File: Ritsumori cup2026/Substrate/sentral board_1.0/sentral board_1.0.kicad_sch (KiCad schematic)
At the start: 9 parts, among them J1 Conn_02x10_Odd_Even, J2 Conn_02x05_Counter_Clockwise, J3 Conn_01x04_Socket, J4 Conn_01x05_Socket, J5 Conn_01x02_Socket, J6 Conn_01x02_Socket, J7 Conn_01x02_Socket, J8 Conn_01x02_Socket, J9 Conn_01x04_Socket

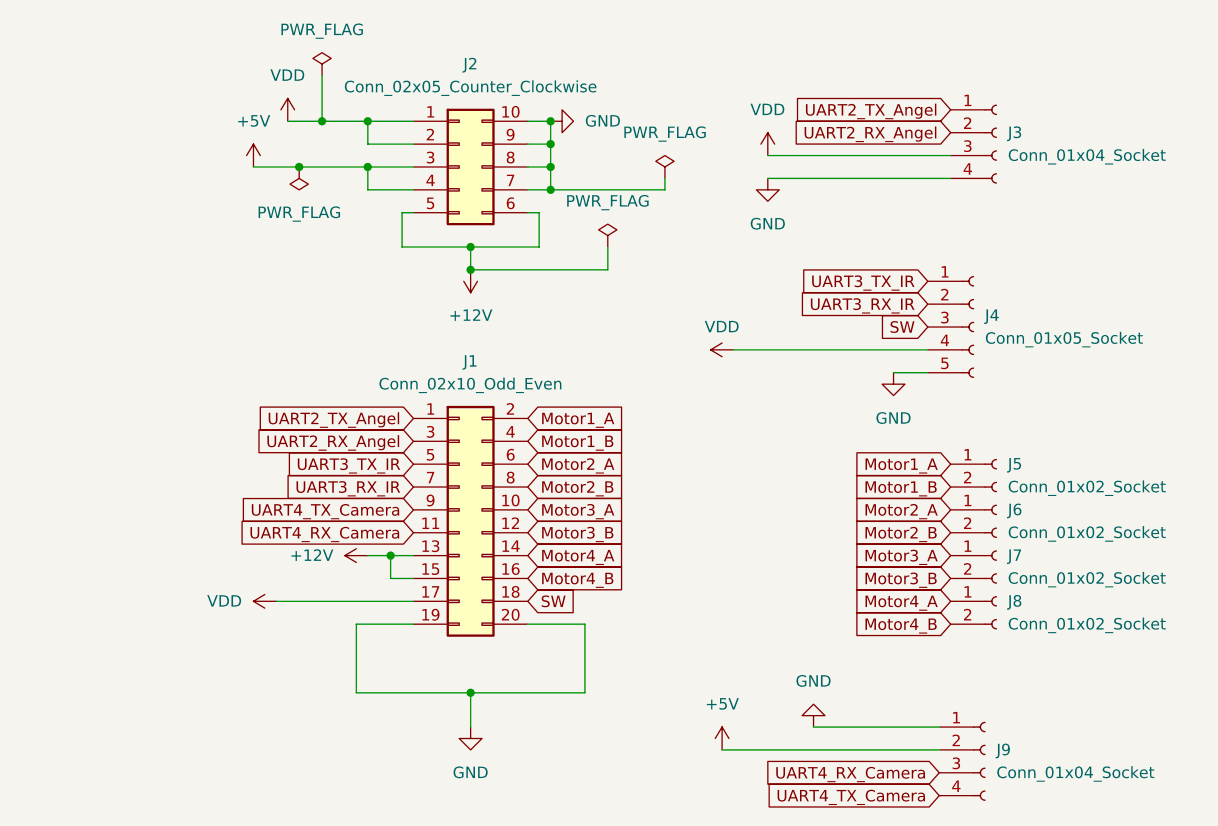
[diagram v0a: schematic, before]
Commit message: Auto Backup: 2026/02/19 18:25:14.96
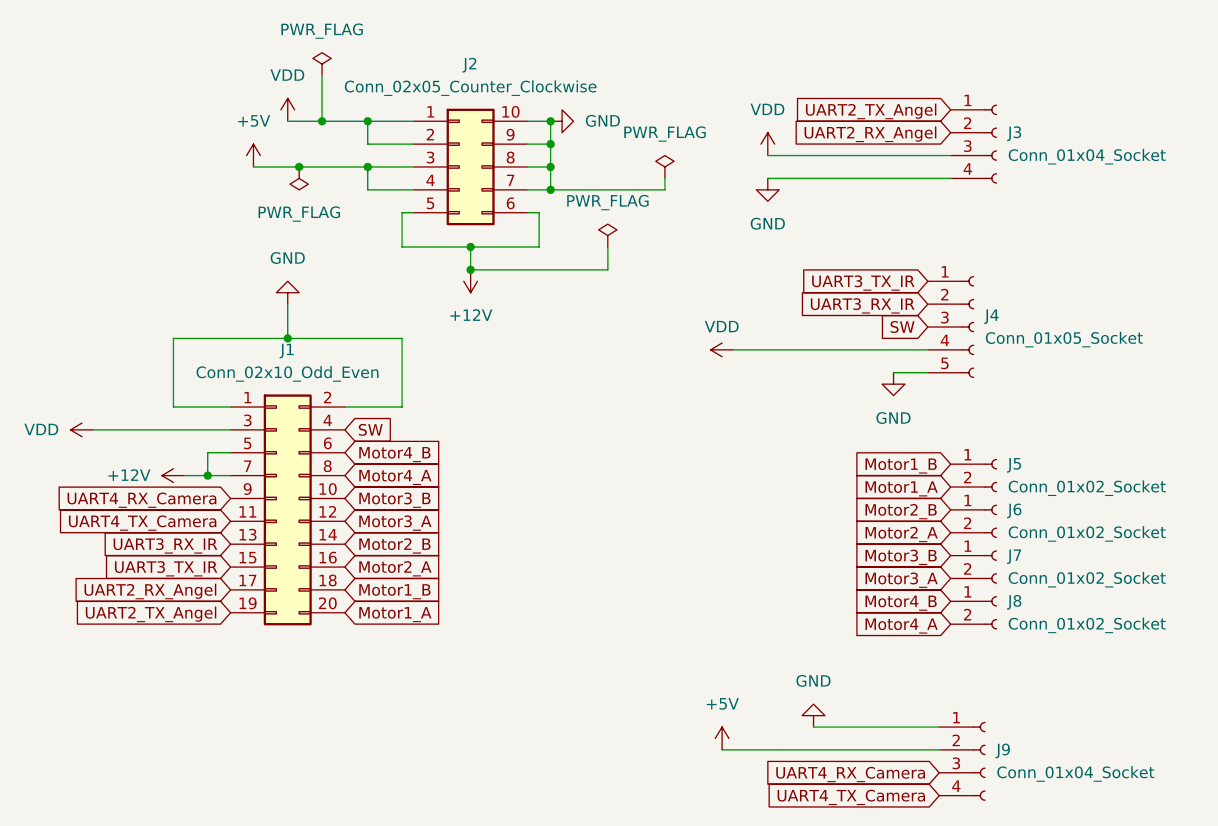
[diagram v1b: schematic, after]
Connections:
- net +12V: now also J1.5 (Pin_5), J1.7 (Pin_7); no longer J1.13 (Pin_13), J1.15 (Pin_15)
- net GND: now also J1.1 (Pin_1), J1.2 (Pin_2); no longer J1.19 (Pin_19), J1.20 (Pin_20)
- net Motor1_A: now also J1.20 (Pin_20), J5.2 (Pin_2); no longer J1.2 (Pin_2), J5.1 (Pin_1)
- net Motor1_B: now also J1.18 (Pin_18), J5.1 (Pin_1); no longer J1.4 (Pin_4), J5.2 (Pin_2)
- net Motor2_A: now also J1.16 (Pin_16), J6.2 (Pin_2); no longer J1.6 (Pin_6), J6.1 (Pin_1)
- net Motor2_B: now also J1.14 (Pin_14), J6.1 (Pin_1); no longer J1.8 (Pin_8), J6.2 (Pin_2)
- net Motor3_A: now also J1.12 (Pin_12), J7.2 (Pin_2); no longer J1.10 (Pin_10), J7.1 (Pin_1)
- net Motor3_B: now also J1.10 (Pin_10), J7.1 (Pin_1); no longer J1.12 (Pin_12), J7.2 (Pin_2)
- net Motor4_A: now also J1.8 (Pin_8), J8.2 (Pin_2); no longer J1.14 (Pin_14), J8.1 (Pin_1)
- net Motor4_B: now also J1.6 (Pin_6), J8.1 (Pin_1); no longer J1.16 (Pin_16), J8.2 (Pin_2)
- net SW: now also J1.4 (Pin_4); no longer J1.18 (Pin_18)
- net UART2_RX_Angel: now also J1.17 (Pin_17); no longer J1.3 (Pin_3)
- net UART2_TX_Angel: now also J1.19 (Pin_19); no longer J1.1 (Pin_1)
- net UART3_RX_IR: now also J1.13 (Pin_13); no longer J1.7 (Pin_7)
- net UART3_TX_IR: now also J1.15 (Pin_15); no longer J1.5 (Pin_5)
- net UART4_RX_Camera: now also J1.9 (Pin_9); no longer J1.11 (Pin_11)
- net UART4_TX_Camera: now also J1.11 (Pin_11); no longer J1.9 (Pin_9)
- net VDD: now also J1.3 (Pin_3); no longer J1.17 (Pin_17)
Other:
- moved on the sheet: J1
